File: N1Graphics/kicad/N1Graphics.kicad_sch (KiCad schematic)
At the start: 3 parts, among them J1 D7 Output, U1 Character_ROM, U2 27C32

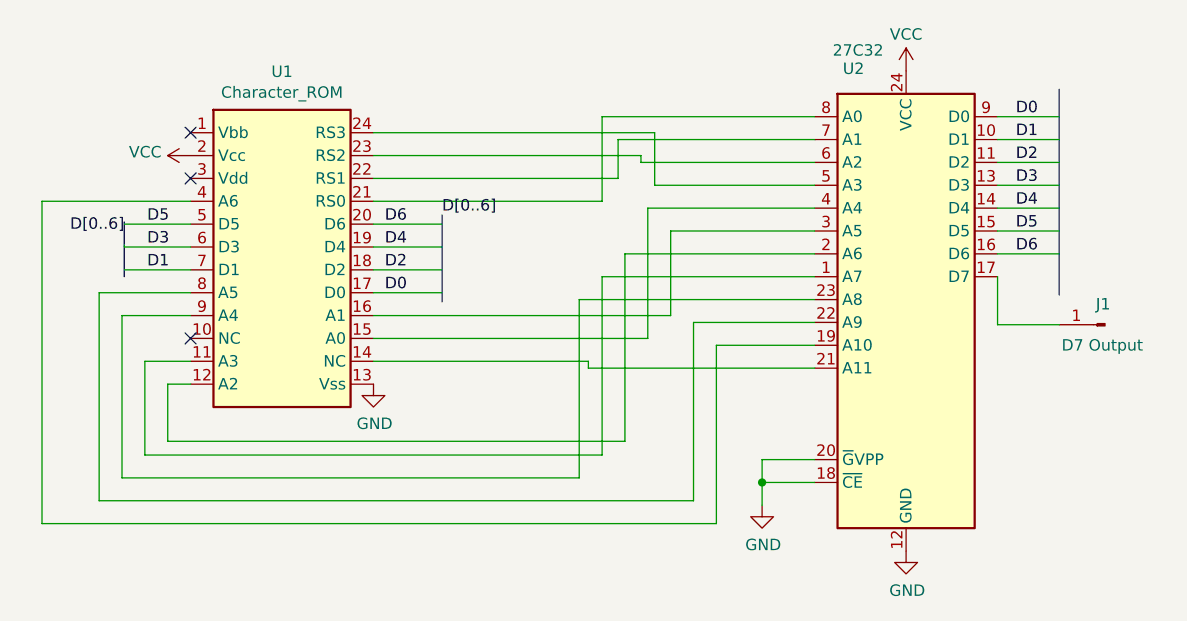
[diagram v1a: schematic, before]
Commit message: Kicad 9 updates
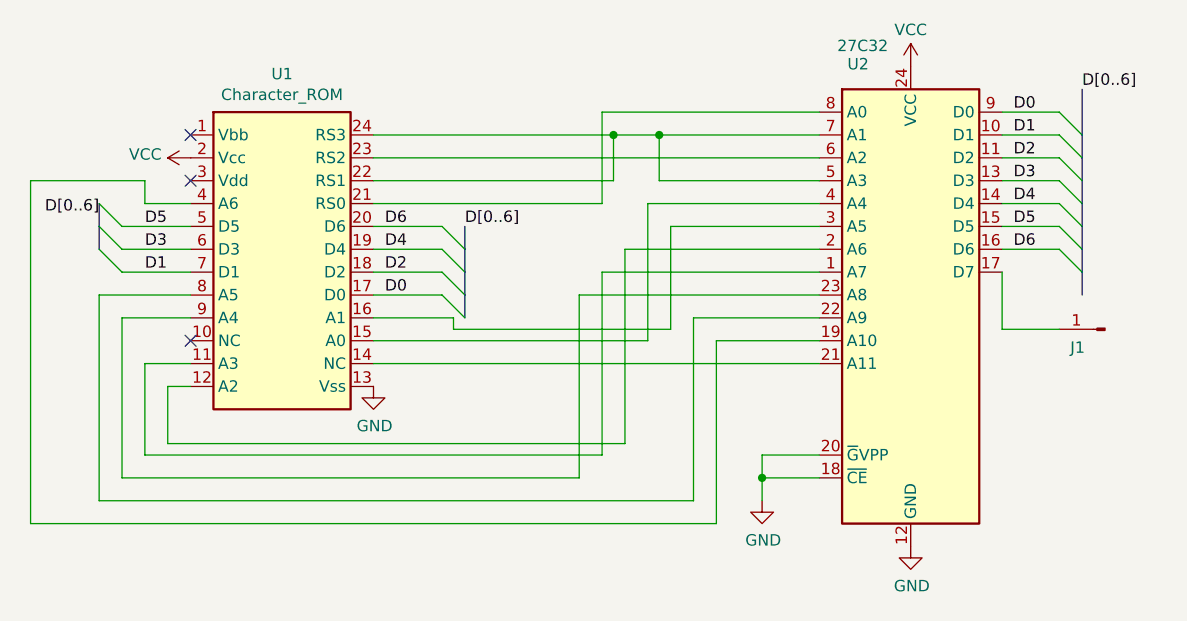
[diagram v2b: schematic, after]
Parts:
- removed J1: D7 Output, Connector_PinHeader_2.54mm:PinHeader_1x01_P2.54mm_Vertical, symbol Connector:Conn_01x01_Male
- added J1: Conn_01x01_Pin, Connector_PinHeader_2.54mm:PinHeader_1x01_P2.54mm_Vertical, symbol Connector:Conn_01x01_Pin
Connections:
- net at U2.17 (D7): now also J1.1 (Pin_1)
- net at U1.24 (RS3), U2.5 (A3): now also U1.22 (RS1), U2.7 (A1)
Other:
- title: N1 Graphics Exapnsion -> N1 Graphics Exapnsion - Kicad 9
- moved on the sheet: U2
